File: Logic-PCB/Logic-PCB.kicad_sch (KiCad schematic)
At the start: 123 parts, among them IC1 74AUP1T87GWH, IC1 MC14027BDR2G, IC10 74LVC1G08FW5-7, IC11 MC14027BDR2G, IC12 TMUX4051PWR, IC13 TMUX4051PWR, IC14 TMUX4051PWR, IC15 TMUX4051PWR, IC16 TMUX4051PWR, IC17 TMUX4051PWR, IC18 TMUX4051PWR, IC19 TMUX4051PWR, IC2 LM555CMX_NOPB, IC3 NLV17SZ74USG, IC4 MC14043BDR2G, IC5 MC14027BDR2G, IC6 MC14027BDR2G, IC7 CD4082BM96, IC8 74LVC1G32GV,125, IC9 TMUX4051PWR, Q1 MMBT2222, Q1 MMBT2907A-7-F, Q10 MMBT2907A-7-F, Q11 MMBT2907A-7-F, Q8 MMBT2907A-7-F, Q9 MMBT2907A-7-F, SW1 SW_Push, SW2 SW_Push, SW3 SW_Push, SW4 SW_Push, SW5 SW_Push, SW6 SW_Push, SW7 SW_Push, SW8 SW_Push, U1 74AHC1G86W5-7

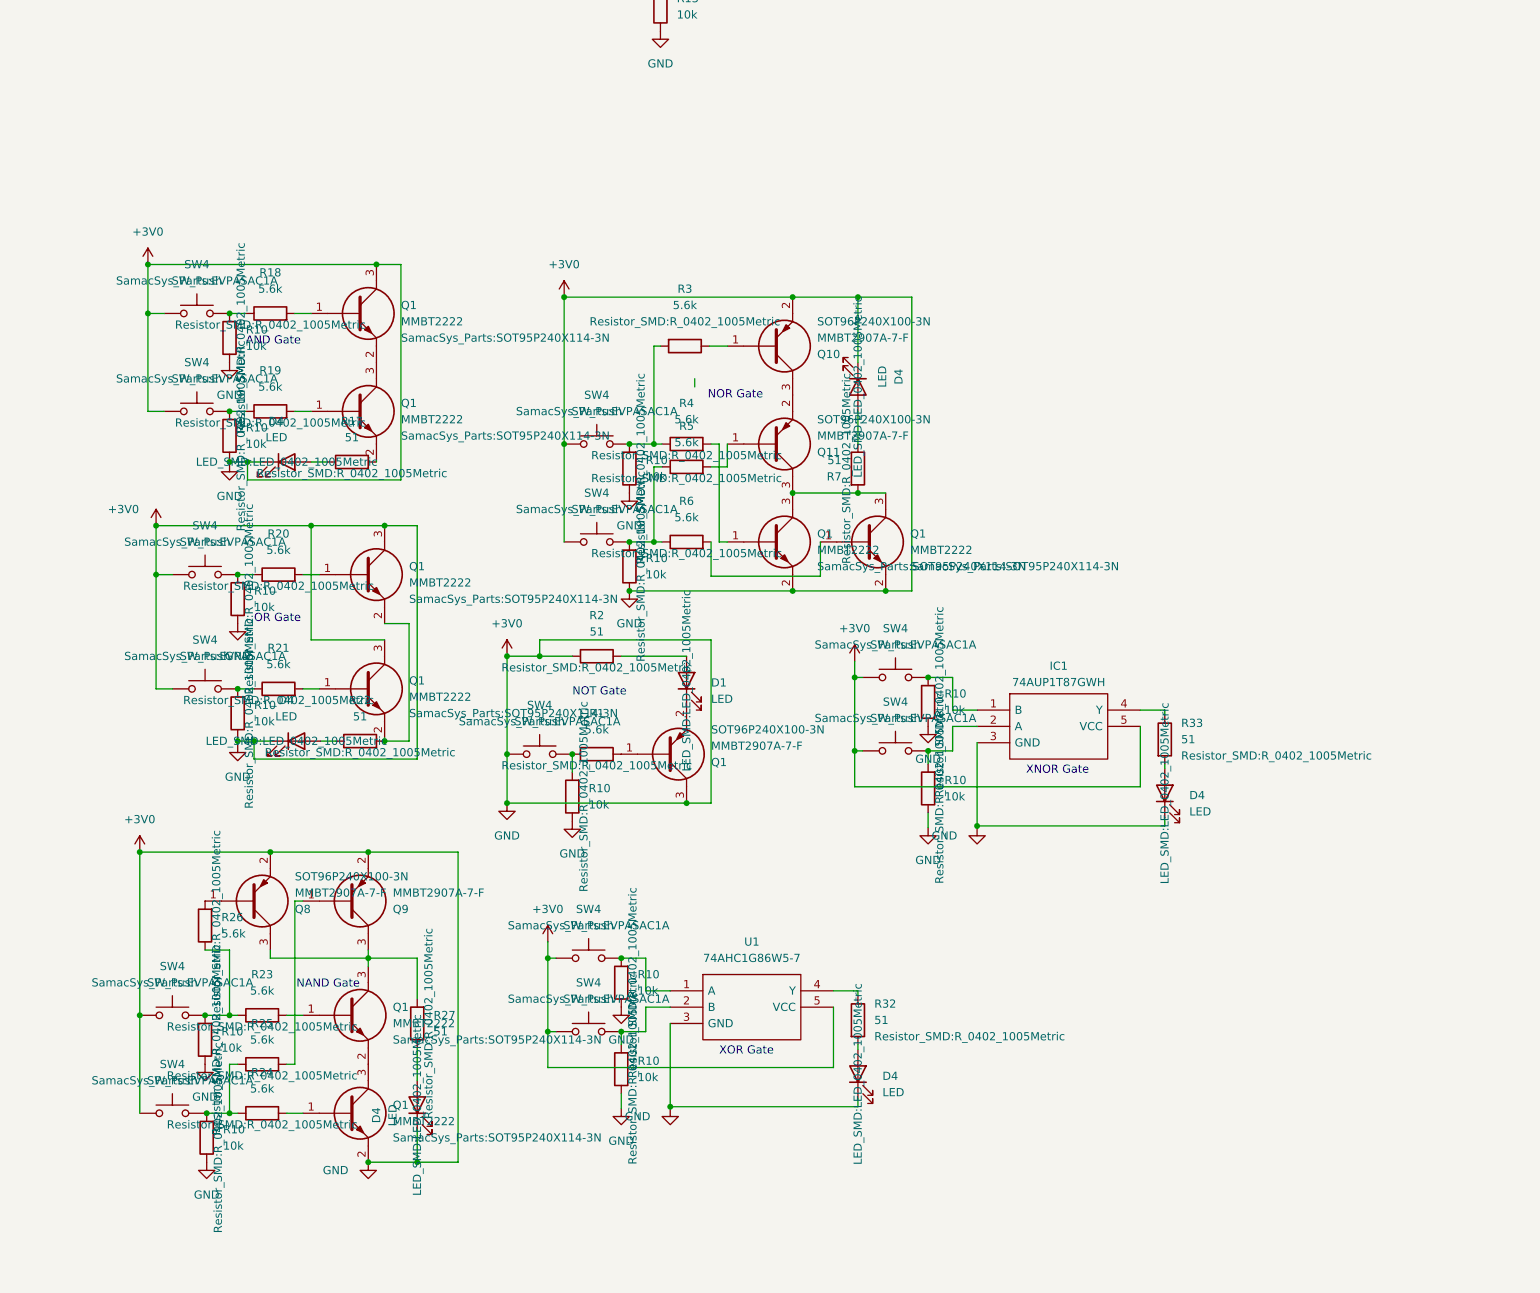
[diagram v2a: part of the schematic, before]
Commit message: Gates
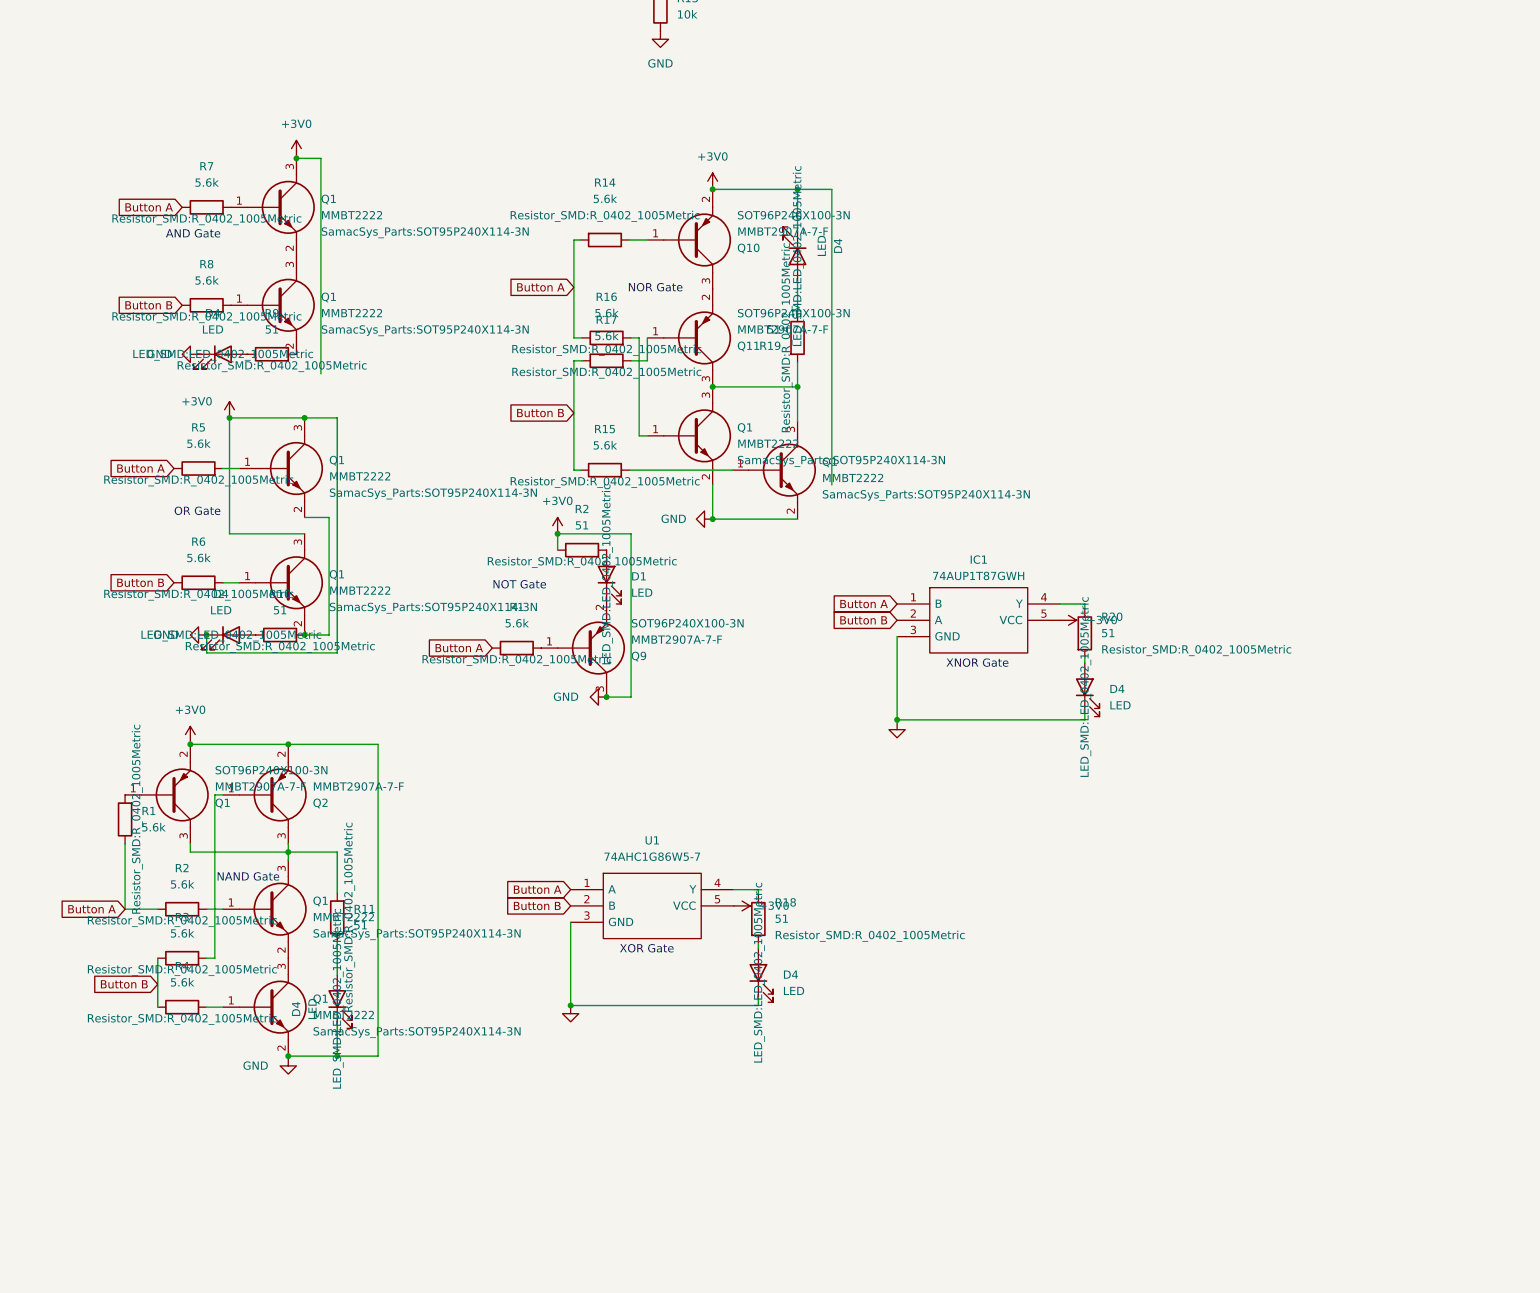
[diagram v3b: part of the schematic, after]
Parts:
- removed D4 (x6): LED, LED_SMD:LED_0402_1005Metric, symbol Device:LED
- removed Q1 (x8): MMBT2222, SamacSys_Parts:SOT95P240X114-3N, symbol SamacSys_Parts:MMBT2222
- removed Q8: MMBT2907A-7-F, SOT96P240X100-3N, symbol SamacSys_Parts:MMBT2907A-7-F
- removed R1, R21, R23, R24, R25, R26: 5.6k, Resistor_SMD:R_0402_1005Metric, symbol Device:R
- removed R10 (x13): 10k, Resistor_SMD:R_0402_1005Metric, symbol Device:R
- removed R2, R22, R27, R32, R33: 51, Resistor_SMD:R_0402_1005Metric, symbol Device:R
- removed SW4 (x13): SW_Push, SamacSys_Parts:EVPASAC1A, symbol Switch:SW_Push
- added D4 (x6): LED, LED_SMD:LED_0402_1005Metric, symbol Device:LED
- added Q1 (x8): MMBT2222, SamacSys_Parts:SOT95P240X114-3N, symbol SamacSys_Parts:MMBT2222
- added Q2: MMBT2907A-7-F, SOT96P240X100-3N, symbol SamacSys_Parts:MMBT2907A-7-F
- added R1 (x2), R14, R15, R16, R2, R8: 5.6k, Resistor_SMD:R_0402_1005Metric, symbol Device:R
- added R10, R11, R2, R9: 51, Resistor_SMD:R_0402_1005Metric, symbol Device:R
- R17, R7: value 51 -> 5.6k
- R18, R19, R20: value 5.6k -> 51
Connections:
- net +3V0: now also Q1.2, Q9.3, D4.1 (K), D4.1 (K), D4.1 (K), D4.1 (K), D4.1 (K), D4.1 (K), Q1.2, Q1.2, Q1.2, Q1.3, Q1.3, Q1.3, Q2.2, R2.1; no longer Q1.3, Q9.2
- net at IC1.4 (Y): now also R20.1
- net Button B: now reaches R17.1
- net Button B: now also IC1.2 (A), R3.1, R4.1, R6.1, U1.2 (B), R15.1, R8.1
- net at R17.2: now also Q11.1
- net Button A: now reaches R5.1
- net Button A: now also IC1.1 (B), R7.1, U1.1 (A), R1.1, R1.1, R14.2, R16.1, R2.1; no longer R6.1
- net at R5.2: now also Q1.1; no longer Q11.1
- net at R18.1: now also U1.4 (Y)
- net at R18.2: now also D4.2 (A)
- net at R3.2: now also Q2.1; no longer R4.1
- net at Q9.1: now also R1.2
- net at R19.1: now also D4.2 (A)
- net at R6.2: now also Q1.1
- net at R7.2: now also Q1.1; no longer Q11.3
- net at Q10.1: now also R14.1; no longer R3.1
- net at Q1.1: now also R1.2
- net at R20.2: now also D4.2 (A)
- net at D1.1 (K): now also Q9.2; no longer Q1.2
- net at D1.2 (A): now also R2.2
- net at R19.2: now also Q11.3, Q1.3, Q1.3
- net at R4.2: now also Q1.1
- new net: Q1.2, Q1.3 (x2)
- new net: Q1.3, Q1.3, Q2.3, R11.2
- new net: D4.2 (A), R11.1
- new net: D4.2 (A), R10.1
- new net: Q1.1, R15.2
- new net: Q1.1, R2.2
- new net: Q1.2, Q1.2, R10.2
- new net: D4.2 (A), R9.1
- new net: Q1.1, R8.2
- new net: Q1.2, R9.2
- new net: Q1.1, R16.2
